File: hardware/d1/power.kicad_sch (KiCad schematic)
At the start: 44 parts, among them U10 BLM15PX601SN1D, U11 TPS7A2033PDBVR, U12 TPS7A2018PDBVR, U13 TPS7A2018PDBVR, U7 TPS7A2018PDBVR, U8 TPS7A2033PDBVR, U9 TPS560430XFDBVR

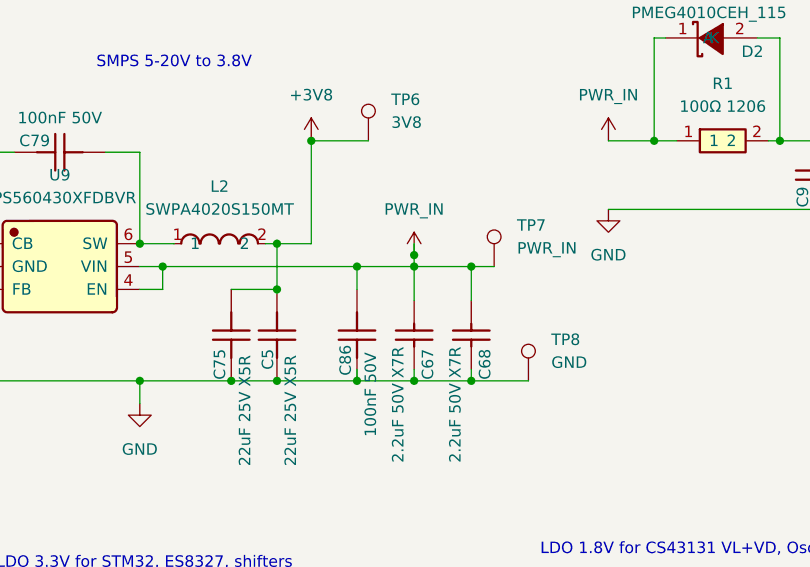
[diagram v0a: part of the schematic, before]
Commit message: Route fixes
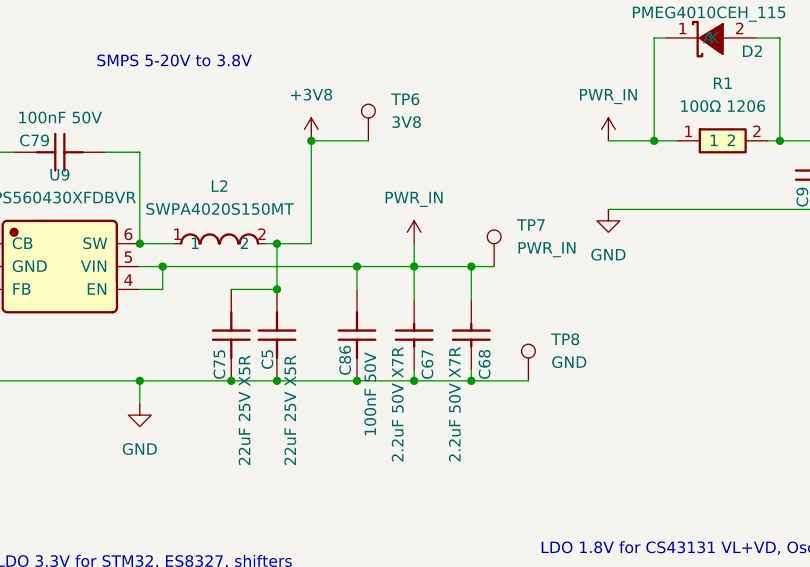
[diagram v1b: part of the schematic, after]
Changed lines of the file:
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@@
 	)
 	(junction
-		(at 87.63 50.8)
+		(at 157.48 44.45)
 		(diameter 0)
 		(color 0 0 0 0)
 	)
 	(junction
-		(at 157.48 44.45)
+		(at 87.63 50.8)
 		(diameter 0)
 		(color 0 0 0 0)
@@
 	)
 	(junction
-		(at 87.63 49.53)
-		(diameter 0)
-		(color 0 0 0 0)
-	)
-	(junction
 		(at 57.15 113.03)
 		(diameter 0)
@@
 	(wire
 		(pts
-			(xy 81.28 62.23) (xy 81.28 63.5)
-		)
-		(stroke
-			(width 0)
-			(type default)
-		)
-	)
-	(wire
-		(pts
-			(xy 87.63 48.26) (xy 87.63 49.53)
-		)
-		(stroke
-			(width 0)
-			(type default)
-		)
-	)
-	(wire
-		(pts
 			(xy 133.35 160.02) (xy 133.35 165.1)
 		)
@@
 	(wire
 		(pts
+			(xy 87.63 50.8) (xy 87.63 54.61)
+		)
+		(stroke
+			(width 0)
+			(type default)
+		)
+	)
+	(wire
+		(pts
 			(xy 24.13 57.15) (xy 34.29 57.15)
 		)
@@
 	(wire
 		(pts
-			(xy 87.63 49.53) (xy 87.63 54.61)
-		)
-		(stroke
-			(width 0)
-			(type default)
-		)
-	)
-	(wire
-		(pts
 			(xy 93.98 62.23) (xy 93.98 63.5)
 		)
@@
 	(wire
 		(pts
+			(xy 87.63 50.8) (xy 96.52 50.8)
+		)
+		(stroke
+			(width 0)
+			(type default)
+		)
+	)
+	(wire
+		(pts
 			(xy 109.22 99.06) (xy 113.03 99.06)
 		)
@@
 	(wire
 		(pts
+			(xy 87.63 48.26) (xy 87.63 50.8)
+		)
+		(stroke
+			(width 0)
+			(type default)
+		)
+	)
+	(wire
+		(pts
 			(xy 142.24 36.83) (xy 147.32 36.83)
 		)
@@
 	(wire
 		(pts
-			(xy 87.63 50.8) (xy 96.52 50.8)
-		)
-		(stroke
-			(width 0)
-			(type default)
-		)
-	)
-	(wire
-		(pts
 			(xy 157.48 36.83) (xy 162.56 36.83)
 		)
@@
 	(symbol
 		(lib_id "power:+5V")
-		(at 87.63 49.53 0)
+		(at 87.63 48.26 0)
 		(unit 1)
 		(body_style 1)
@@
 		(fields_autoplaced yes)
 		(property "Reference" "#PWR022"
-			(at 87.63 53.34 0)
+			(at 87.63 52.07 0)
 			(hide yes)
 			(show_name no)
@@
 		)
 		(property "Value" "PWR_IN"
-			(at 87.63 44.45 0)
+			(at 87.63 43.18 0)
 			(show_name no)
 			(do_not_autoplace no)
@@
 		)
 		(property "Footprint" ""
-			(at 87.63 49.53 0)
+			(at 87.63 48.26 0)
 			(hide yes)
 			(show_name no)
@@
 		)
 		(property "Datasheet" ""
-			(at 87.63 49.53 0)
+			(at 87.63 48.26 0)
 			(hide yes)
 			(show_name no)
@@
 		)
 		(property "Description" "Power symbol creates a global label with name \"+5V\""
-			(at 87.63 49.53 0)
+			(at 87.63 48.26 0)
 			(hide yes)
 			(show_name no)
